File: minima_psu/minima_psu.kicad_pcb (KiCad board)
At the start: 2 copper layers, 78 x 90 mm, 28 parts, among them J1 Screw_Terminal_01x03, J2 Screw_Terminal_01x02, J3 Screw_Terminal_01x03, J4 Screw_Terminal_01x03, J5 Screw_Terminal_01x03, J6 Screw_Terminal_01x03

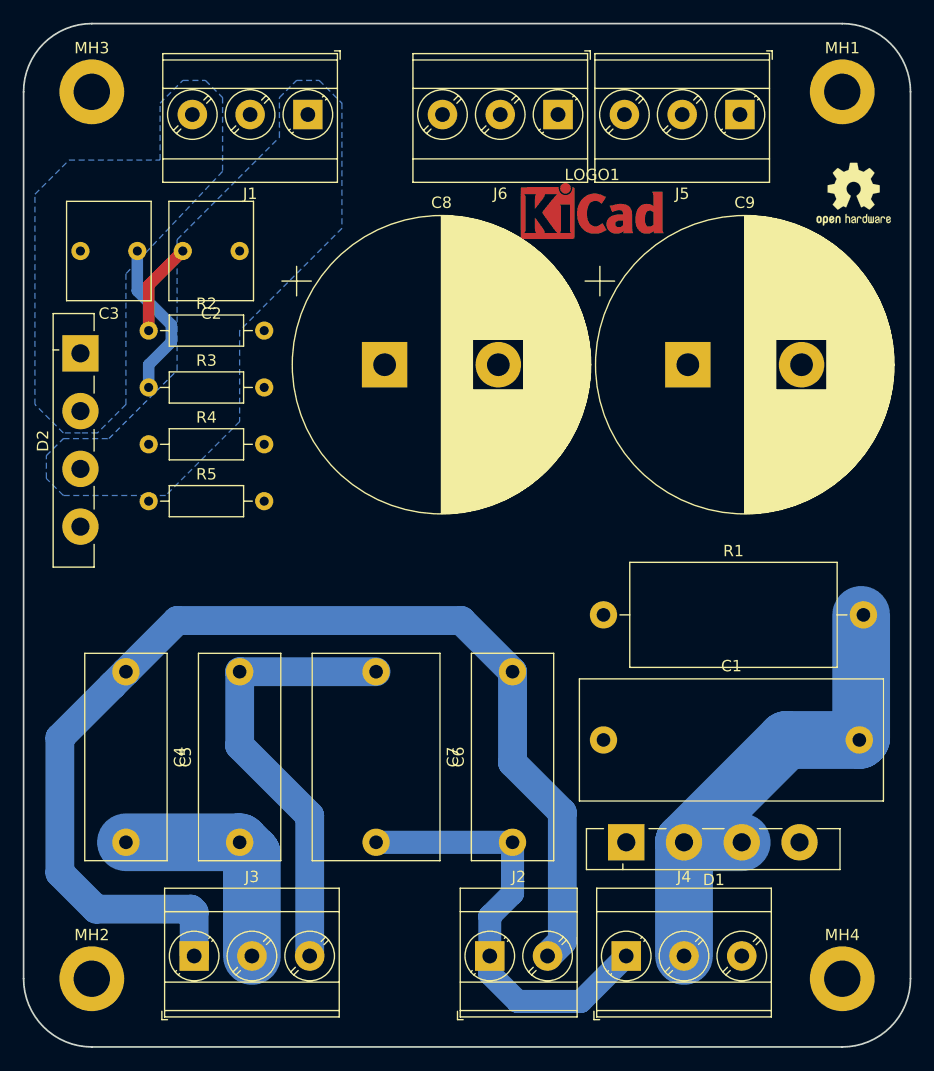
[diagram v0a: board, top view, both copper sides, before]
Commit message: WIP: Component routing & placement
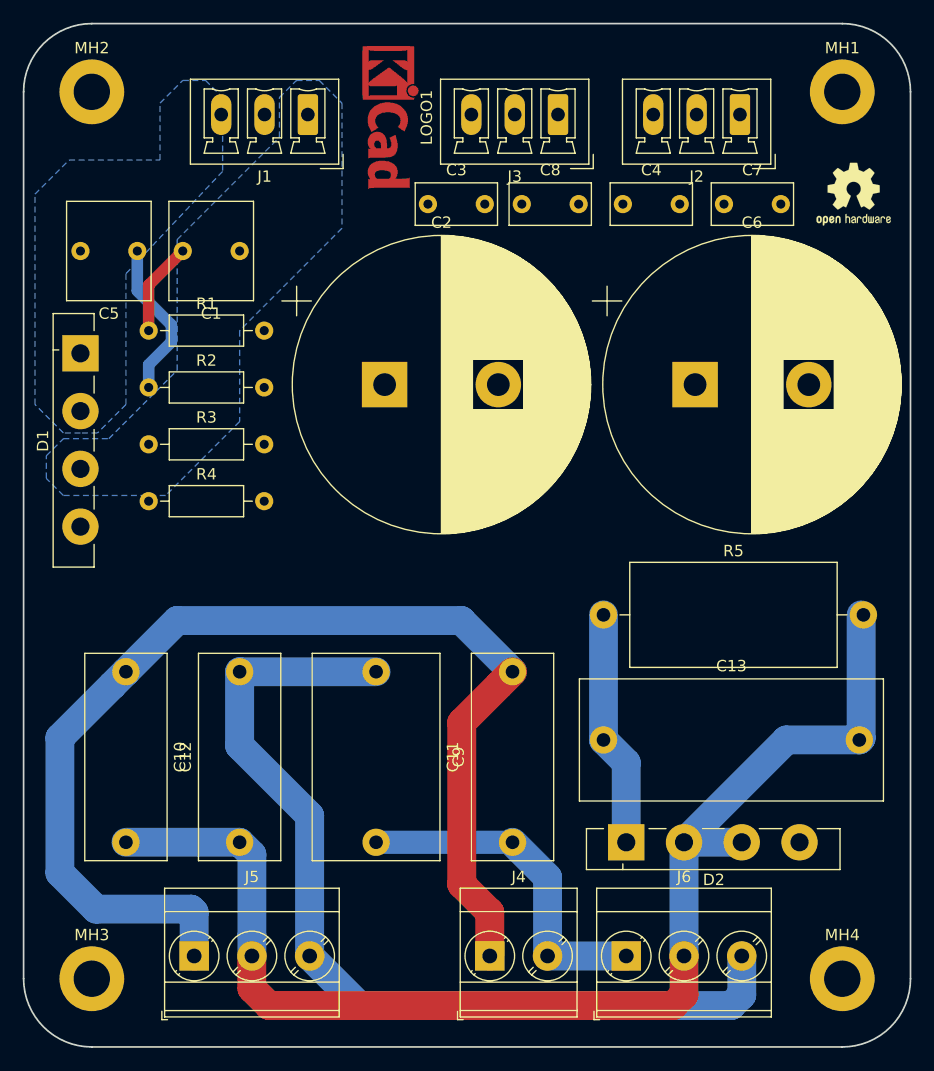
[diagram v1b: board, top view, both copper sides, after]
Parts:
- removed the J4 at (148.2, 151.8)
- added C3: 100n, Capacitor_THT:C_Rect_L7.0mm_W3.5mm_P5.00mm, F.Cu at (130.8, 85.7)
- added C4: 100n, Capacitor_THT:C_Rect_L7.0mm_W3.5mm_P5.00mm, F.Cu at (148.0, 85.7)
- added C7: 100n, Capacitor_THT:C_Rect_L7.0mm_W3.5mm_P5.00mm, F.Cu at (156.8, 85.7)
- added C8: 100n, Capacitor_THT:C_Rect_L7.0mm_W3.5mm_P5.00mm, F.Cu at (139.1, 85.7)
- added J2: psupply, Connector_Phoenix_MC:PhoenixContact_MCV_1,5_3-G-3.81_1x03_P3.81mm_Vertical, F.Cu at (158.2, 77.8)
- J1: value Screw_Terminal_01x03 -> power; footprint TerminalBlock_Phoenix:TerminalBlock_Phoenix_MKDS-3-3-5.08_1x03_P5.08mm_Horizontal -> Connector_Phoenix_MC:PhoenixContact_MCV_1,5_3-G-3.81_1x03_P3.81mm_Vertical
- J3: value Screw_Terminal_01x03 -> psupply; footprint TerminalBlock_Phoenix:TerminalBlock_Phoenix_MKDS-3-3-5.08_1x03_P5.08mm_Horizontal -> Connector_Phoenix_MC:PhoenixContact_MCV_1,5_3-G-3.81_1x03_P3.81mm_Vertical
- J4: renamed from J2; value Screw_Terminal_01x02 -> switch
- J5: value Screw_Terminal_01x03 -> ac_in
- J6: value Screw_Terminal_01x03 -> transformer
- moved J5 88.2 mm to (110.2, 151.8), turned to 0 degrees
- moved J3 80.6 mm to (142.2, 77.8), turned to 180 degrees
- moved J6 74.2 mm to (148.2, 151.8), turned to 0 degrees
- moved LOGO1 20.2 mm to (127.0, 78.1), turned to 270 degrees
- moved C6 1.86 mm to (154.3, 101.6)
- moved C2 1.75 mm to (127.0, 101.6)
- renumbered C2 to C1, C4 to C10, C7 to C11, C5 to C12, C1 to C13, C8 to C2, C3 to C5, C9 to C6, C6 to C9, D2 to D1, D1 to D2, MH3 to MH2, MH2 to MH3, R2 to R1, R3 to R2, R4 to R3, R5 to R4, R1 to R5
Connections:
- C11 pad 2: Net-(C6-Pad1) -> Net-(C11-Pad2)
- C9 pad 1: Net-(C6-Pad1) -> Net-(C11-Pad2)
- J3 pad 1: /ac_l -> /vcc
- J3 pad 2: Earth_Protective -> GNDPWR
- J3 pad 3: /ac_n -> /vee
- J4 pad 1: Net-(C6-Pad1) -> /ac_l
- J4 pad 2: /ac_l -> Net-(C11-Pad2)
- J5 pad 1: /vcc -> /ac_l
- J5 pad 2: GNDPWR -> Earth_Protective
- J5 pad 3: /vee -> /ac_n
- J6 pad 1: /vcc -> Net-(C11-Pad2)
- J6 pad 2: GNDPWR -> Earth_Protective
- J6 pad 3: /vee -> /ac_n
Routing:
- net Earth_Protective: track 65.7 -> 111.0 mm
- net /ac_n: track 39.6 -> 83.2 mm
- net Net-(C6-Pad1): track 39.1 -> 0.00 mm
- net Net-(C11-Pad2): track 0.00 -> 30.2 mm
- net GNDPWR: track 0.00 -> 20.8 mm
- net /ac_l: track 102.3 -> 102.8 mm
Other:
- net class ac_prot: trace_width 5.08 -> 2.54
- net class dc_p: trace_width 5.08 -> 2.54
